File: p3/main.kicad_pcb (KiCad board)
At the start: 2 copper layers, 54 x 23 mm, 15 parts, among them P1 CONN_XT60, P4 CONN_XT60, Q1 BSS138, U1 AUIPS7111S, U2 LM3480-5.0, U3 74LVC1G08

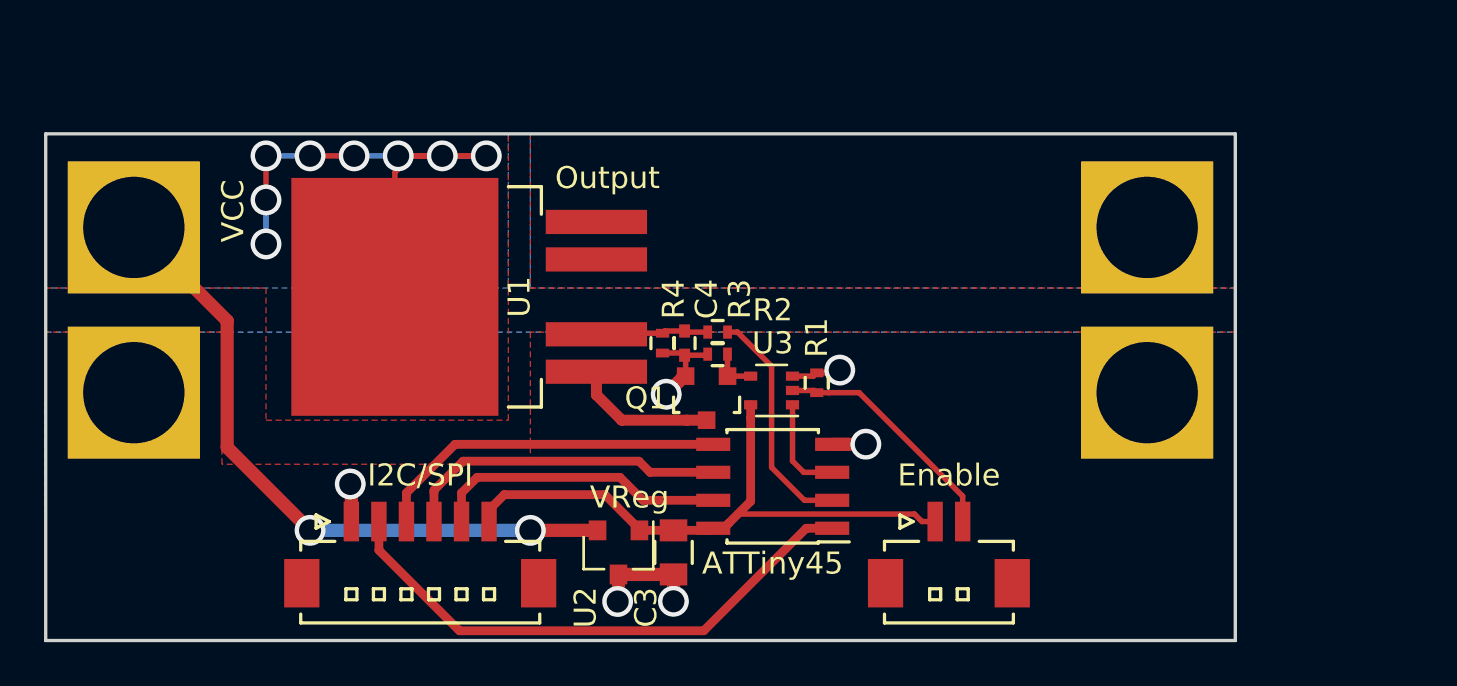
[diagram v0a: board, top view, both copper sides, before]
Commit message: test
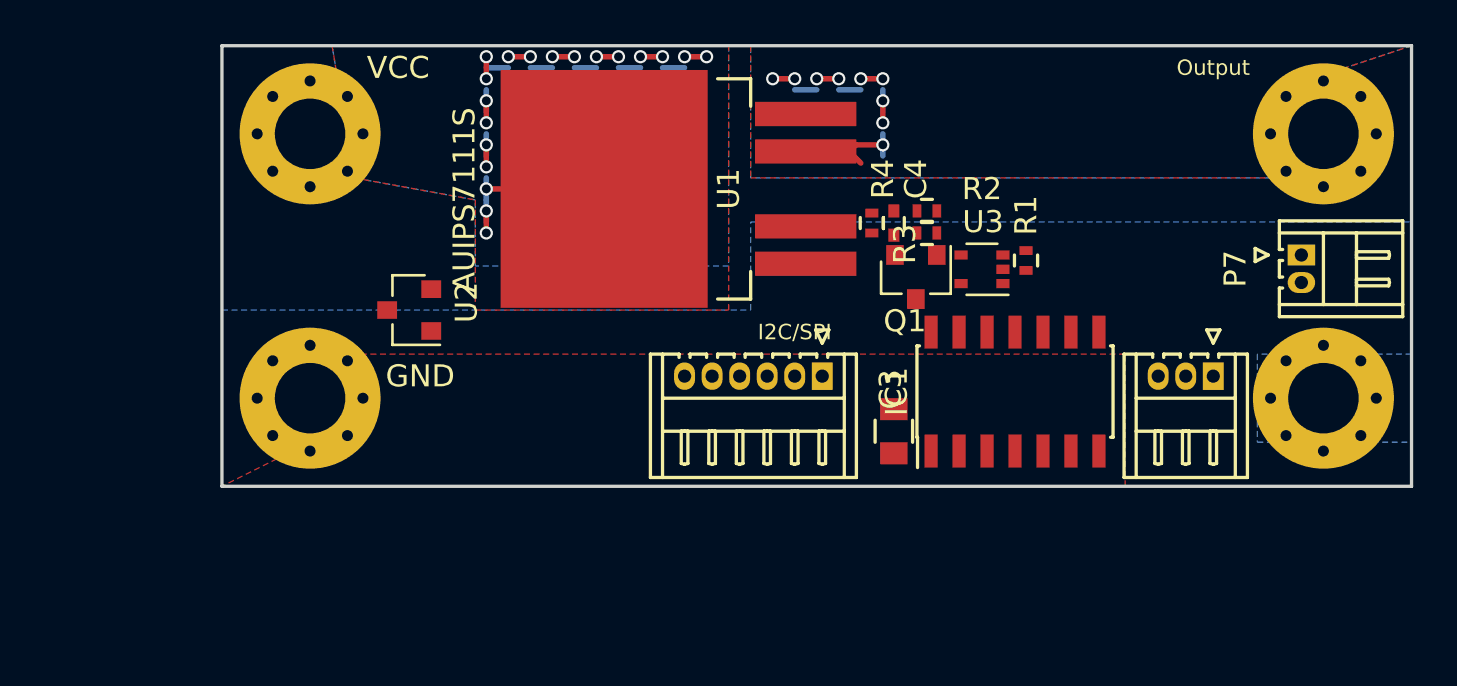
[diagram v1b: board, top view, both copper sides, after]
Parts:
- removed ATTiny45: ATTINY45-P, Housings_SOIC:SOIC-8_3.9x4.9mm_Pitch1.27mm
- removed Enable: CONN_01X02, Connectors_Hirose:Hirose_DF13C-02P-1.25V_02x1.25mm_Straight
- removed I2C/SPI: CONN_01X06, Connectors_Hirose:Hirose_DF13C-06P-1.25V_06x1.25mm_Straight
- added IC1: ATTINY84-S, Housings_SOIC:SOIC-14_3.9x8.7mm_Pitch1.27mm, F.Cu at (157.0, 92.7)
- added P2: CONN_01X06, Connectors_Hirose:Hirose_DF13-06P-1.25DS_06x1.25mm_Angled, F.Cu at (148.2, 92.0)
- added P3: CONN_01X03, Connectors_Hirose:Hirose_DF13-03P-1.25DS_03x1.25mm_Angled, F.Cu at (166.0, 92.0)
- added P5: CONN_01X01, Mounting_Holes:MountingHole_3.2mm_M3_Pad_Via, F.Cu at (171.0, 81.0)
- added P6: CONN_01X01, Mounting_Holes:MountingHole_3.2mm_M3_Pad_Via, F.Cu at (125.0, 93.0)
- added P7: CONN_01X02, Connectors_Hirose:Hirose_DF13-02P-1.25DS_02x1.25mm_Angled, F.Cu at (170.0, 86.5)
- P1, P4: value CONN_XT60 -> CONN_01X01; footprint KiCad-MDH-Connectors:XT60 -> Mounting_Holes:MountingHole_3.2mm_M3_Pad_Via; moved to F.Cu
- moved U2 14.5 mm to (129.5, 89.0), turned to 180 degrees
- moved C3 11.4 mm to (151.5, 94.5), turned to 90 degrees
- moved P1 11.3 mm to (125.0, 81.0)
- moved U3 11.0 mm to (155.5, 87.2)
- moved R1 11.0 mm to (157.5, 86.8)
- moved Q1 11.0 mm to (152.5, 87.5), turned to 270 degrees
- moved R2 11.0 mm to (153.0, 85.5)
- moved R3 11.0 mm to (153.0, 84.5), turned to 180 degrees
- moved C4 11.0 mm to (151.5, 85.0)
- moved R4 11.0 mm to (150.5, 85.0)
- moved U1 10.7 mm to (147.5, 83.5)
- moved P4 8.94 mm to (171.0, 93.0)
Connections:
- net +3V3 renamed +5V
- P1 pad 1: GND -> VCC
- R3 pad 1: /Ifb -> /Current_Feedback
- R3 pad 2: Net-(IC1-Pad2) -> /Ifb
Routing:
- net VCC: track 54.2 -> 5.35 mm, vias 10 -> 1
- net +5V: track 28.0 -> 0.00 mm
- net (no net): track 0.00 -> 26.0 mm, vias 0 -> 26
- net /RESET: track 25.3 -> 0.00 mm
- net /SDA/MOSI: track 16.1 -> 0.00 mm
- net /MISO: track 14.9 -> 0.00 mm
- net GND: track 14.8 -> 0.00 mm, vias 6 -> 0
- net /SCL/SCK: track 13.4 -> 0.00 mm
- net /ENB2: track 10.9 -> 0.00 mm
- net Net-(IC1-Pad2): track 10.6 -> 0.00 mm
- net /IN: track 6.53 -> 0.00 mm
- net /Ifb: track 5.13 -> 0.00 mm
- net /Out: track 0.00 -> 4.95 mm, vias 0 -> 1
- net /ENB1: track 4.57 -> 0.00 mm
- net Net-(Q1-Pad1): track 2.05 -> 0.00 mm
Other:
- board size 54 x 23 mm -> 54 x 20 mm
- board text added: "AUIPS7111S"
- board text added: "GND"
- board text added: "I2C/SPI"
- board text removed: "VReg"
